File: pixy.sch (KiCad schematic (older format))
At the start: 1 part, among them J15 Conn_01x10

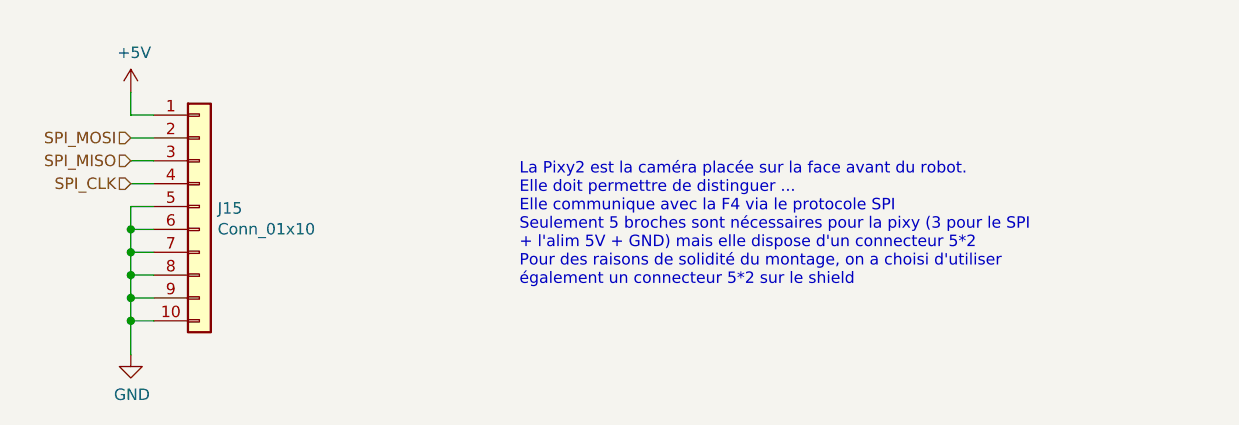
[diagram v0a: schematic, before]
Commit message: Add files via upload
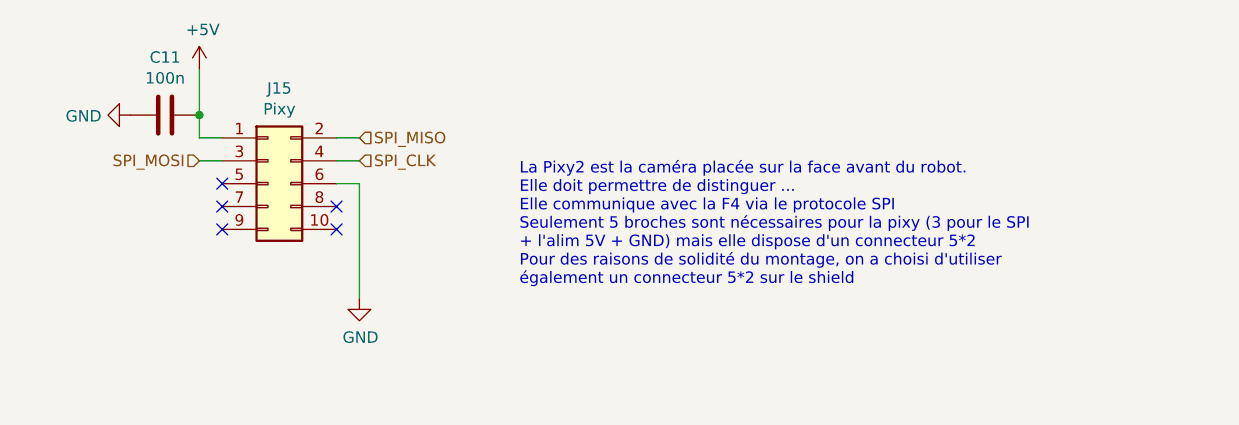
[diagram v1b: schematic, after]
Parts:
- removed J15: Conn_01x10, symbol Connector_Generic:Conn_01x10
- added C11: 100n, Capacitor_SMD:C_0805_2012Metric_Pad1.15x1.40mm_HandSolder, symbol Device:C
- added J15: Pixy, Connector_JST:JST_PHD_B10B-PHDSS_2x05_P2.00mm_Vertical, symbol Connector_Generic:Conn_02x05_Odd_Even
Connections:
- net +5V: now also C11.1, J15.1 (Pin_1)
- net GND: now also C11.2, J15.6 (Pin_6)
- net SPI_CLK: now also J15.4 (Pin_4)
- net SPI_MISO: now also J15.2 (Pin_2)
- net SPI_MOSI: now also J15.3 (Pin_3)
- no-connect marks 0 -> 5
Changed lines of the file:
@@
 EESchema Schematic File Version 4
-LIBS:kicad_master-cache
 EELAYER 30 0
 EELAYER END
 $Descr A4 11693 8268
 encoding utf-8
-Sheet 21 22
+Sheet 19 21
 Title ""
 Date ""
@@
 Comment4 ""
 $EndDescr
-Text HLabel 5000 2650 0    50   Input ~ 0
+Text HLabel 5300 2750 0    50   Input ~ 0
 SPI_MOSI
-Text HLabel 5000 2750 0    50   Input ~ 0
+Text HLabel 6000 2650 2    50   Input ~ 0
 SPI_MISO
-Text HLabel 5000 2850 0    50   Input ~ 0
+Text HLabel 6000 2750 2    50   Input ~ 0
 SPI_CLK
 $Comp
 L power:+5V #PWR0122
 U 1 1 5E8459BC
-P 5000 2450
-F 0 "#PWR0122" H 5000 2300 50  0001 C CNN
-F 1 "+5V" H 5015 2623 50  0000 C CNN
-F 2 "" H 5000 2450 50  0001 C CNN
-F 3 "" H 5000 2450 50  0001 C CNN
-	1    5000 2450
-	1    0    0    -1
-$EndComp
-$Comp
-L power:GND #PWR0123
-U 1 1 5E84620F
-P 5000 3600
-F 0 "#PWR0123" H 5000 3350 50  0001 C CNN
-F 1 "GND" H 5005 3427 50  0000 C CNN
-F 2 "" H 5000 3600 50  0001 C CNN
-F 3 "" H 5000 3600 50  0001 C CNN
-	1    5000 3600
-	1    0    0    -1
-$EndComp
-$Comp
-L Connector_Generic:Conn_01x10 J15
-U 1 1 5E86FCF9
-P 5300 2950
-F 0 "J15" H 5380 2942 50  0000 L CNN
-F 1 "Conn_01x10" H 5380 2851 50  0000 L CNN
-F 2 "" H 5300 2950 50  0001 C CNN
-F 3 "~" H 5300 2950 50  0001 C CNN
-	1    5300 2950
+P 5300 2350
+F 0 "#PWR0122" H 5300 2200 50  0001 C CNN
+F 1 "+5V" H 5315 2523 50  0000 C CNN
+F 2 "" H 5300 2350 50  0001 C CNN
+F 3 "" H 5300 2350 50  0001 C CNN
+	1    5300 2350
 	1    0    0    -1
 $EndComp
 Wire Wire Line
-	5000 2450 5000 2550
+	5300 2650 5400 2650
 Wire Wire Line
-	5000 2550 5100 2550
+	5300 2750 5400 2750
 Wire Wire Line
-	5100 2950 5000 2950
+	6000 2650 5900 2650
 Wire Wire Line
-	5000 2950 5000 3050
-Wire Wire Line
-	5100 3050 5000 3050
-Connection ~ 5000 3050
-Wire Wire Line
-	5000 3050 5000 3150
-Wire Wire Line
-	5100 3150 5000 3150
-Connection ~ 5000 3150
-Wire Wire Line
-	5000 3150 5000 3250
-Wire Wire Line
-	5100 3250 5000 3250
-Connection ~ 5000 3250
-Wire Wire Line
-	5000 3250 5000 3350
-Wire Wire Line
-	5100 3350 5000 3350
-Connection ~ 5000 3350
-Wire Wire Line
-	5000 3350 5000 3450
-Wire Wire Line
-	5100 3450 5000 3450
-Connection ~ 5000 3450
-Wire Wire Line
-	5000 3450 5000 3600
-Wire Wire Line
-	5100 2650 5000 2650
-Wire Wire Line
-	5000 2750 5100 2750
-Wire Wire Line
-	5100 2850 5000 2850
+	5900 2750 6000 2750
 Text Notes 6700 3300 0    50   ~ 0
 La Pixy2 est la caméra placée sur la face avant du robot.\nElle doit permettre de distinguer ...\nElle communique avec la F4 via le protocole SPI\nSeulement 5 broches sont nécessaires pour la pixy (3 pour le SPI\n+ l'alim 5V + GND) mais elle dispose d'un connecteur 5*2\nPour des raisons de solidité du montage, on a choisi d'utiliser\négalement un connecteur 5*2 sur le shield
+$Comp
+L Device:C C11
+U 1 1 5E88A20B
+P 5150 2550
+F 0 "C11" V 4898 2550 50  0000 C CNN
+F 1 "100n" V 4989 2550 50  0000 C CNN
+F 2 "Capacitor_SMD:C_0805_2012Metric_Pad1.15x1.40mm_HandSolder" H 5188 2400 50  0001 C CNN
+F 3 "~" H 5150 2550 50  0001 C CNN
+	1    5150 2550
+	0    1    1    0
+$EndComp
+$Comp
+L power:GND #PWR01
+U 1 1 5E88AA1B
+P 5000 2550
+F 0 "#PWR01" H 5000 2300 50  0001 C CNN
+F 1 "GND" V 5005 2422 50  0000 R CNN
+F 2 "" H 5000 2550 50  0001 C CNN
+F 3 "" H 5000 2550 50  0001 C CNN
+	1    5000 2550
+	0    1    1    0
+$EndComp
+$Comp
+L Connector_Generic:Conn_02x05_Odd_Even J15
+U 1 1 5E88593F
+P 5600 2850
+F 0 "J15" H 5650 3267 50  0000 C CNN
+F 1 "Pixy" H 5650 3176 50  0000 C CNN
+F 2 "Connector_JST:JST_PHD_B10B-PHDSS_2x05_P2.00mm_Vertical" H 5600 2850 50  0001 C CNN
+F 3 "~" H 5600 2850 50  0001 C CNN
+	1    5600 2850
+	1    0    0    -1
+$EndComp
+Wire Wire Line
+	5900 2850 6000 2850
+Wire Wire Line
+	6000 2850 6000 3350
+$Comp
+L power:GND #PWR026
+U 1 1 5E88CD14
+P 6000 3350
+F 0 "#PWR026" H 6000 3100 50  0001 C CNN
+F 1 "GND" H 6005 3177 50  0000 C CNN
+F 2 "" H 6000 3350 50  0001 C CNN
+F 3 "" H 6000 3350 50  0001 C CNN
+	1    6000 3350
+	1    0    0    -1
+$EndComp
+NoConn ~ 5900 2950
+NoConn ~ 5900 3050
+NoConn ~ 5400 3050
+NoConn ~ 5400 2950
+NoConn ~ 5400 2850
+Wire Wire Line
+	5300 2350 5300 2550
+Connection ~ 5300 2550
+Wire Wire Line
+	5300 2550 5300 2650
 $EndSCHEMATC

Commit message: avancement général du routage
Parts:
- C11: symbol Device:C -> shield_etage2-rescue:C-Device
- J15: symbol Connector_Generic:Conn_02x05_Odd_Even -> shield_etage2-rescue:Conn_02x05_Odd_Even-Connector_Generic
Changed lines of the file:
@@
 SPI_CLK
 $Comp
-L power:+5V #PWR0122
+L shield_etage2-rescue:+5V-power #PWR0122
 U 1 1 5E8459BC
 P 5300 2350
@@
 La Pixy2 est la caméra placée sur la face avant du robot.\nElle doit permettre de distinguer ...\nElle communique avec la F4 via le protocole SPI\nSeulement 5 broches sont nécessaires pour la pixy (3 pour le SPI\n+ l'alim 5V + GND) mais elle dispose d'un connecteur 5*2\nPour des raisons de solidité du montage, on a choisi d'utiliser\négalement un connecteur 5*2 sur le shield
 $Comp
-L Device:C C11
+L shield_etage2-rescue:C-Device C11
 U 1 1 5E88A20B
 P 5150 2550
@@
 $EndComp
 $Comp
-L power:GND #PWR01
+L shield_etage2-rescue:GND-power #PWR01
 U 1 1 5E88AA1B
 P 5000 2550
@@
 $EndComp
 $Comp
-L Connector_Generic:Conn_02x05_Odd_Even J15
+L shield_etage2-rescue:Conn_02x05_Odd_Even-Connector_Generic J15
 U 1 1 5E88593F
 P 5600 2850
@@
 	6000 2850 6000 3350
 $Comp
-L power:GND #PWR026
+L shield_etage2-rescue:GND-power #PWR026
 U 1 1 5E88CD14
 P 6000 3350
